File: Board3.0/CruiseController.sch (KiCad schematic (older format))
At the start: 55 parts, among them J1 USB_B_Micro, J2 Conn_02x09_Top_Bottom, U1 ADG884, U3 TLV9064IRTER, U5 MIC5225, U6 MCP2562-E-MF, U7 STM32L433CCUx, Y1 32.768

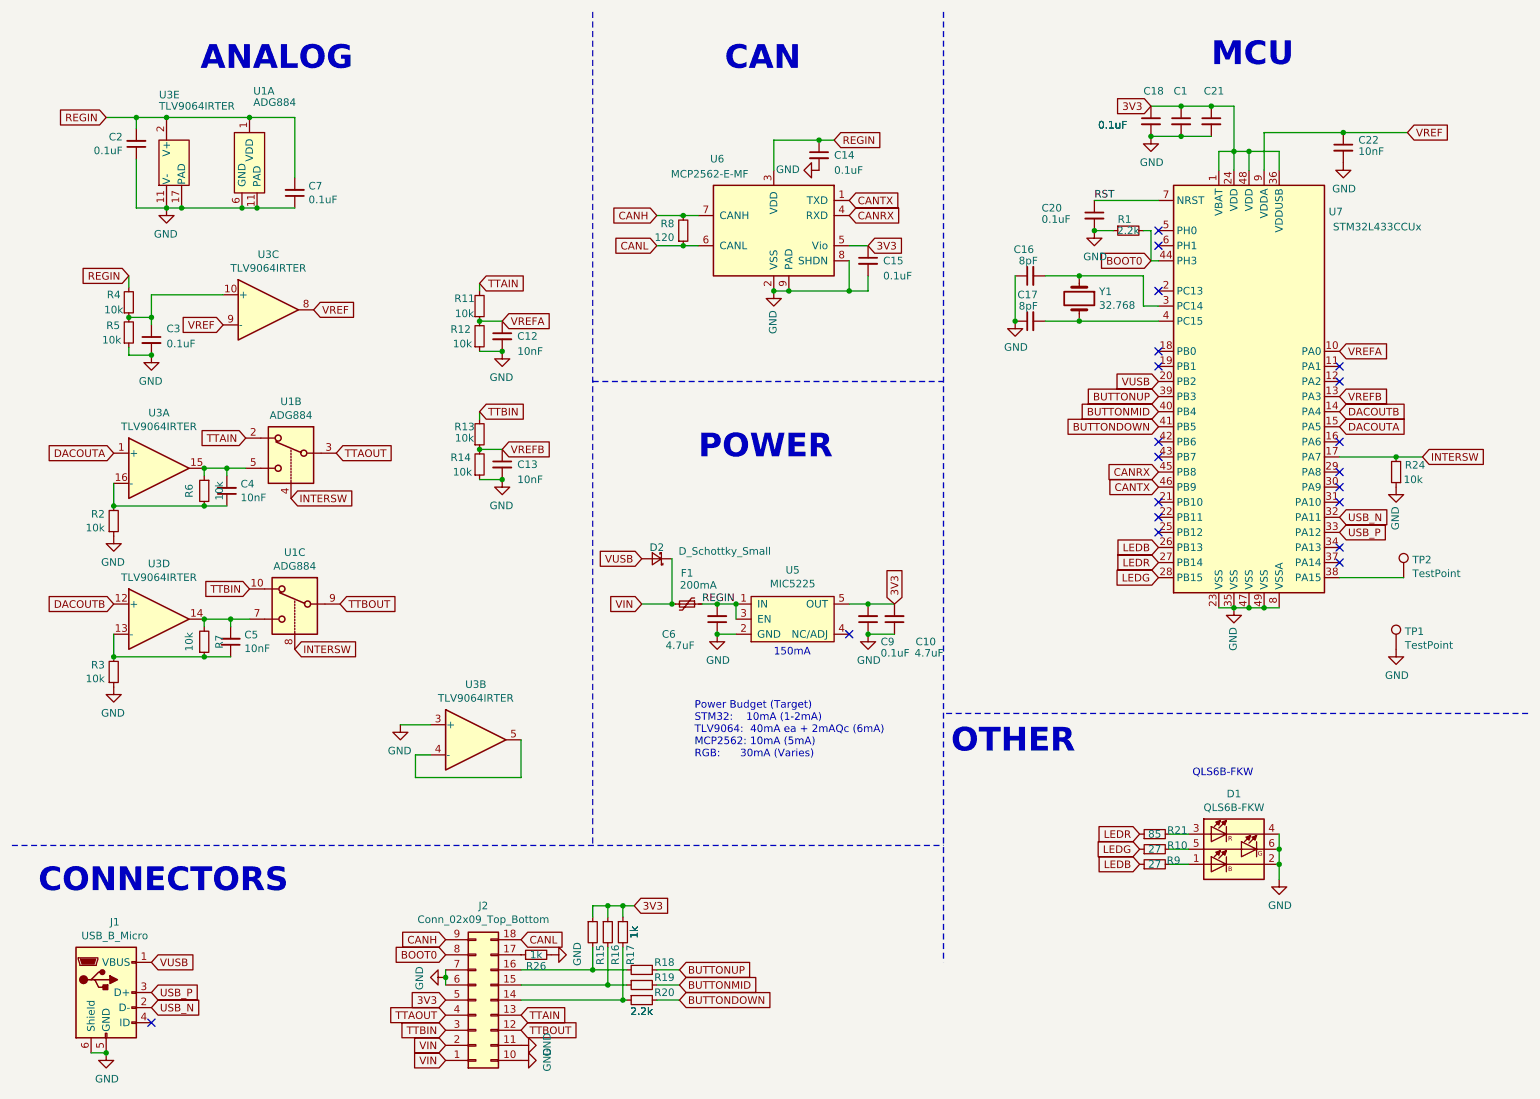
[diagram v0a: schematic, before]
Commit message: Update V3
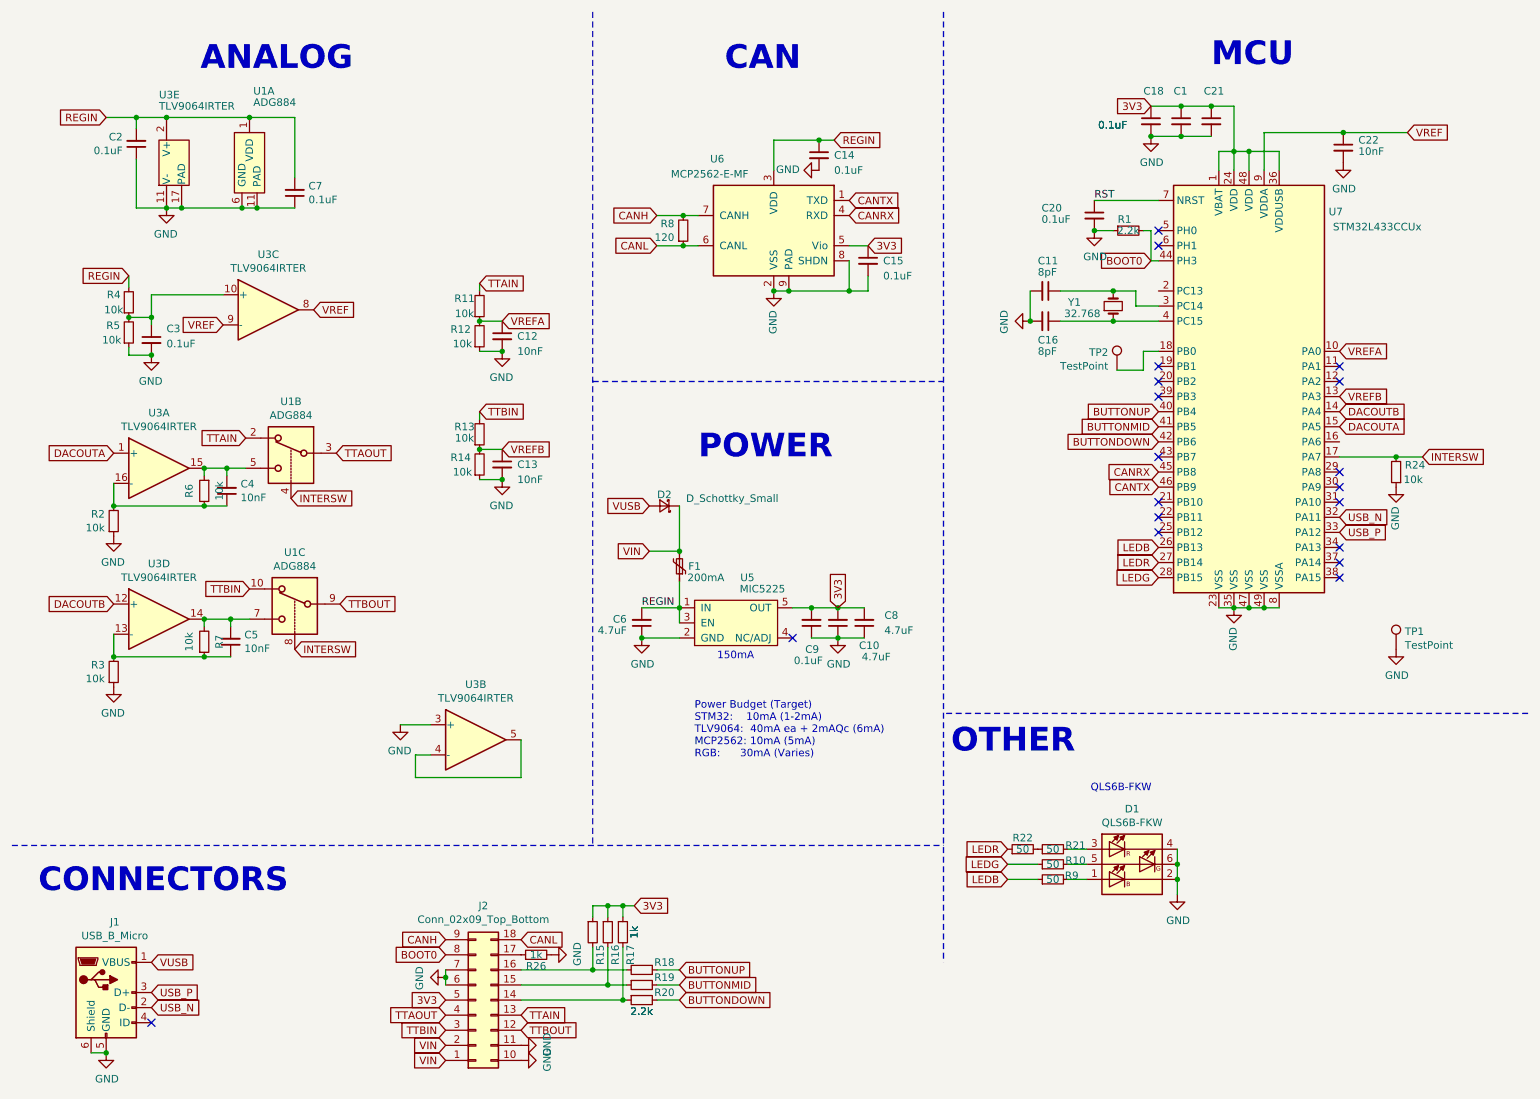
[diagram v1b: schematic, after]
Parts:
- removed C17: 8pF, Capacitor_SMD:C_0603_1608Metric, symbol Device:C_Small
- removed Y1: 32.768, Crystal:Crystal_SMD_G8-2Pin_3.2x1.5mm, symbol Device:Crystal
- added C11: 8pF, Capacitor_SMD:C_0603_1608Metric, symbol Device:C_Small
- added C8: 4.7uF, Capacitor_SMD:C_0805_2012Metric, symbol Device:C_Small
- added R22: 50, Resistor_SMD:R_0603_1608Metric, symbol Device:R_Small
- added Y1: 32.768, Crystal:Crystal_SMD_G8-2Pin_3.2x1.5mm, symbol Device:Crystal_Small
- R10, R9: value 27 -> 50
- R21: value 85 -> 50
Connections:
- net 3V3: now also C8.2
- net BUTTONDOWN: now also U7.42 (PB6); no longer U7.41 (PB5)
- net BUTTONMID: now also U7.41 (PB5); no longer U7.40 (PB4)
- net BUTTONUP: now also U7.40 (PB4); no longer U7.39 (PB3)
- net GND: now also C16.2, C11.2, C8.1; no longer C16.1
- net LEDR: now also R22.1; no longer R21.1
- net VUSB: no longer U7.20 (PB2)
- net at U7.18 (PB0): now also TP2.1
- net at U7.3 (PC14): now also C11.1, Y1.2; no longer C16.2
- net at U7.38 (PA15): no longer TP2.1
- net at U7.4 (PC15): now also C16.1, Y1.1
- new net: R21.1, R22.2
- no-connect marks 20 -> 19
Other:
- moved on the sheet: C10, C6, C9, D1, D2, F1, R10, R21, R9, TP2, U5
